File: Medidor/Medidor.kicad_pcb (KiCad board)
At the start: 2 copper layers, 59.9 x 47.1 mm, 52 parts, among them J1 TC2030-CTX-TAG_CONECT, SW1 Rotary_Encoder_Switch, SW2 SW_DPST_x2, U1 INA219-INA, U10 spacer, U2 Serial, U3 2450AT18D0100, U4 Fiducial, U5 Fiducial, U6 Fiducial, U7 spacer, U8 spacer, U9 spacer, X1 32MHz

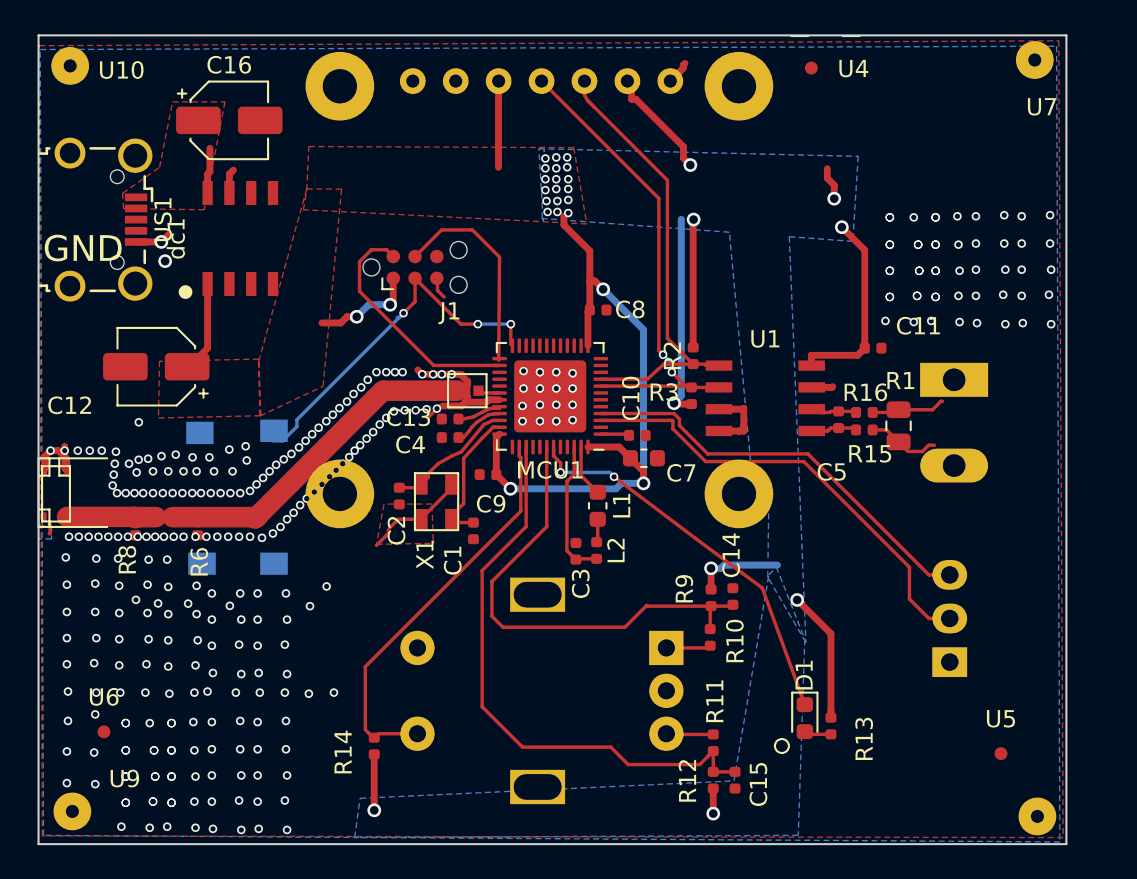
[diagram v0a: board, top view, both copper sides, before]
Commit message: replacement again and again and again
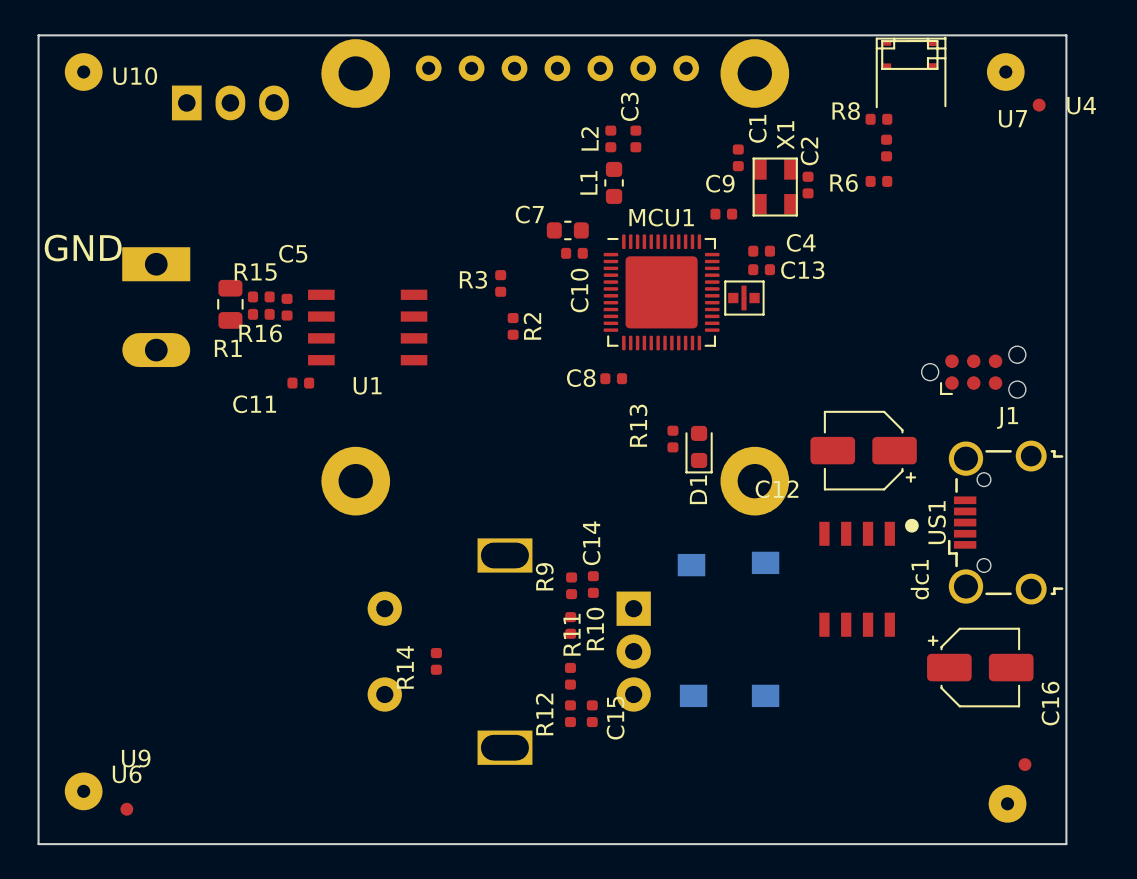
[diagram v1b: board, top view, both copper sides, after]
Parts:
- moved U2 55.1 mm to (92.2, 92.2), turned to 0 degrees
- moved US1 55.0 mm to (139.4, 116.6), turned to 90 degrees
- moved U3 54.2 mm to (132.7, 90.2), turned to 0 degrees
- moved C16 54.1 mm to (138.4, 125.1)
- moved R8 49.4 mm to (132.5, 93.2), turned to 180 degrees
- moved R7 47.3 mm to (133.0, 94.8), turned to 90 degrees
- moved Screw_Terminal 47.0 mm to (90.4, 101.6)
- moved R6 44.5 mm to (132.5, 96.8), turned to 180 degrees
- moved C12 41.5 mm to (131.6, 112.5)
- moved dc1 41.1 mm to (131.3, 120.0), turned to 180 degrees
- moved R1 39.6 mm to (94.7, 103.9), turned to 90 degrees
- moved R15 36.0 mm to (96.5, 103.5), turned to 0 degrees
- moved R16 35.6 mm to (96.5, 104.5), turned to 0 degrees
- moved C11 33.4 mm to (98.8, 108.5), turned to 0 degrees
- moved J1 33.1 mm to (138.0, 107.9)
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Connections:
- MCU1 pad 14: Net-(MCU1-Pad14) -> RC3
- MCU1 pad 15: Net-(MCU1-Pad15) -> RC2
- MCU1 pad 16: Net-(MCU1-Pad16) -> RC1
- MCU1 pad 20: Net-(MCU1-Pad20) -> LEDMCU
- MCU1 pad 38: RC3 -> Net-(MCU1-Pad38)
- MCU1 pad 39: RC2 -> Net-(MCU1-Pad39)
- MCU1 pad 42: RC1 -> Net-(MCU1-Pad42)
- MCU1 pad 43: LEDMCU -> Net-(MCU1-Pad43)
- SW2 pad 1: GND -> nRESET
- SW2 pad 2: nRESET -> GND
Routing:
- net +3V3: track 111.4 -> 0.00 mm, vias 32 -> 0
- net RC2: track 34.0 -> 0.00 mm
- net SDA: track 29.3 -> 0.00 mm, vias 2 -> 0
- net SCL: track 27.6 -> 0.00 mm
- net RC1: track 27.4 -> 0.00 mm
- net /TX: track 26.5 -> 0.00 mm
- net GND: track 25.2 -> 0.00 mm, vias 285 -> 0
- net /RX: track 24.4 -> 0.00 mm
- net RC3: track 23.6 -> 0.00 mm
- net LEDMCU: track 22.9 -> 0.00 mm, vias 2 -> 0
- net nRESET: track 21.7 -> 0.00 mm, vias 5 -> 0
- net Net-(Fil1-Pad3): track 19.7 -> 0.00 mm
- net SWDIO: track 14.1 -> 0.00 mm
- net SWDCLK: track 12.2 -> 0.00 mm
- net Net-(C3-Pad2): track 8.18 -> 0.00 mm
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- removed copper zone on B.Cu, net +3V3
- removed copper zone on F.Cu, net +3V3
- removed copper zone on F.Cu, net +5V
- removed copper zone on B.Cu, net GND
- removed copper zone on F.Cu, net GND
